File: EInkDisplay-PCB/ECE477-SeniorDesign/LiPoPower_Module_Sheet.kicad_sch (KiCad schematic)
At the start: 18 parts, among them J6 Battery Connector, U2 MCP73871, U4 TPS63060, U5 BQ27441-G1

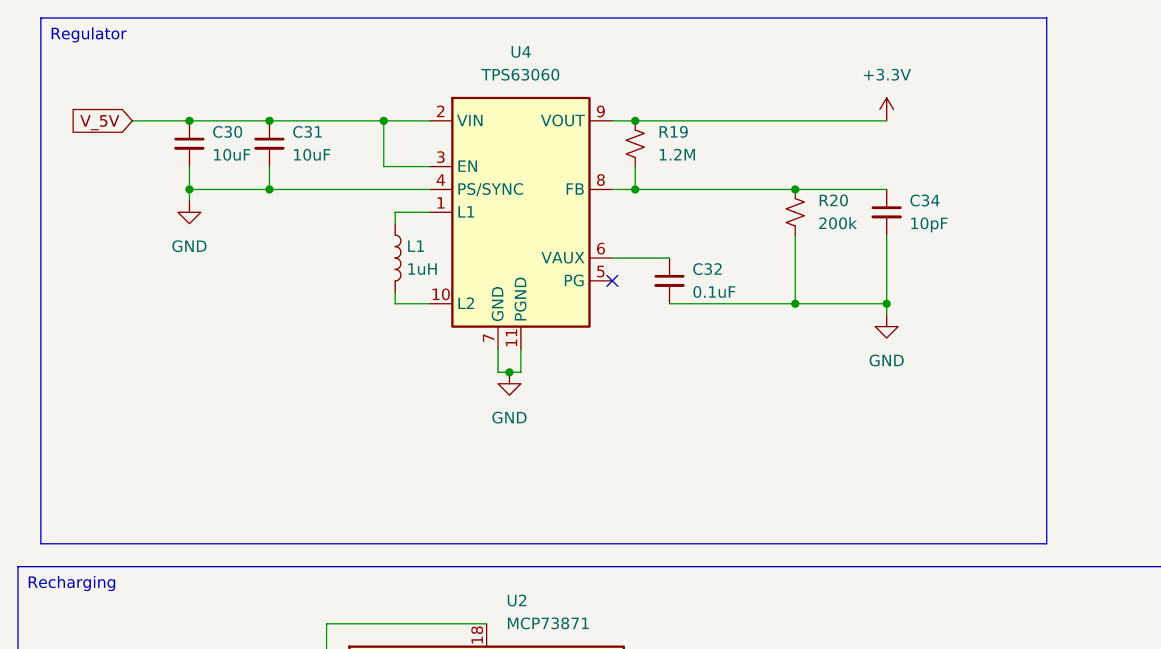
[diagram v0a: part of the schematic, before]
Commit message: Update LiPoPower_Module_Sheet.kicad_sch
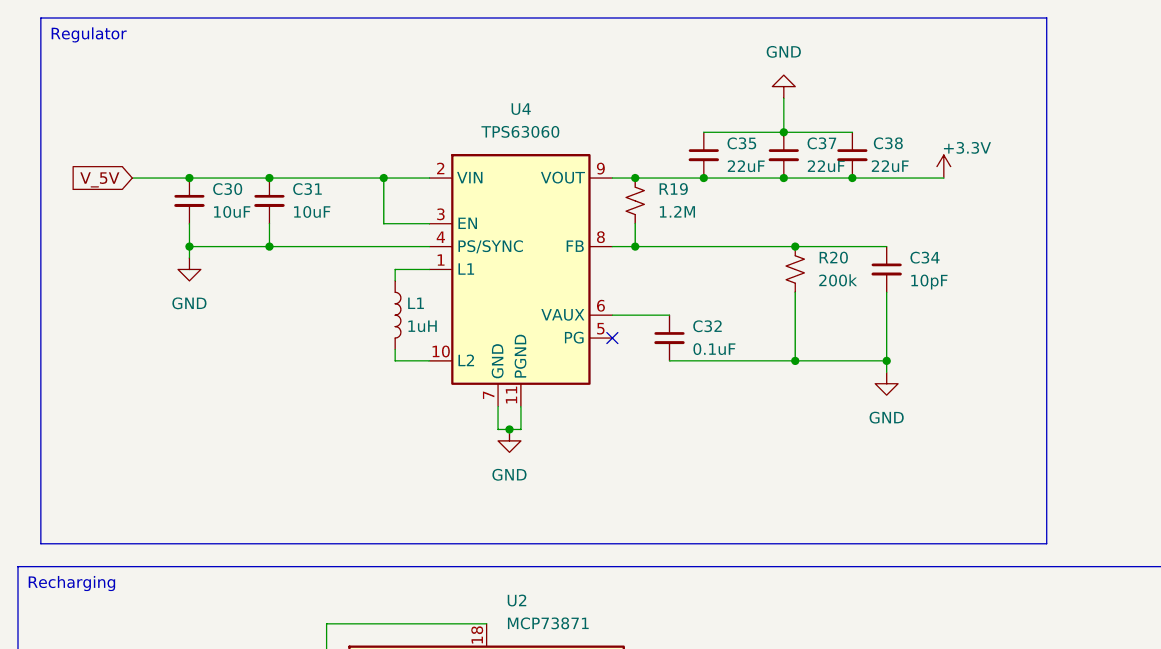
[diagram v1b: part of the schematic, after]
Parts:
- added C35, C37, C38: 22uF, symbol Device:C_Small
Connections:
- net +3.3V: now also C35.2, C37.2, C38.2
- net GND: now also C35.1, C37.1, C38.1
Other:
- moved on the sheet: C30, C31, C32, C34, L1, R19, R20, U4
